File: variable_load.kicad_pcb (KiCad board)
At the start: 2 copper layers, 76.2 x 51 mm, 63 parts, among them J1 Conn_01x04, J2 LEMO, J3 Conn_01x02, J4 GS3, J5 Conn_01x04, J6 Conn_01x04, J7 Conn_01x04, Q1 NTD4858N, U1 DAC5578, U2 LM324, U3 TLV1117-33, U4 PCA9306, U5 adafruit_ft232h, U6 APD123

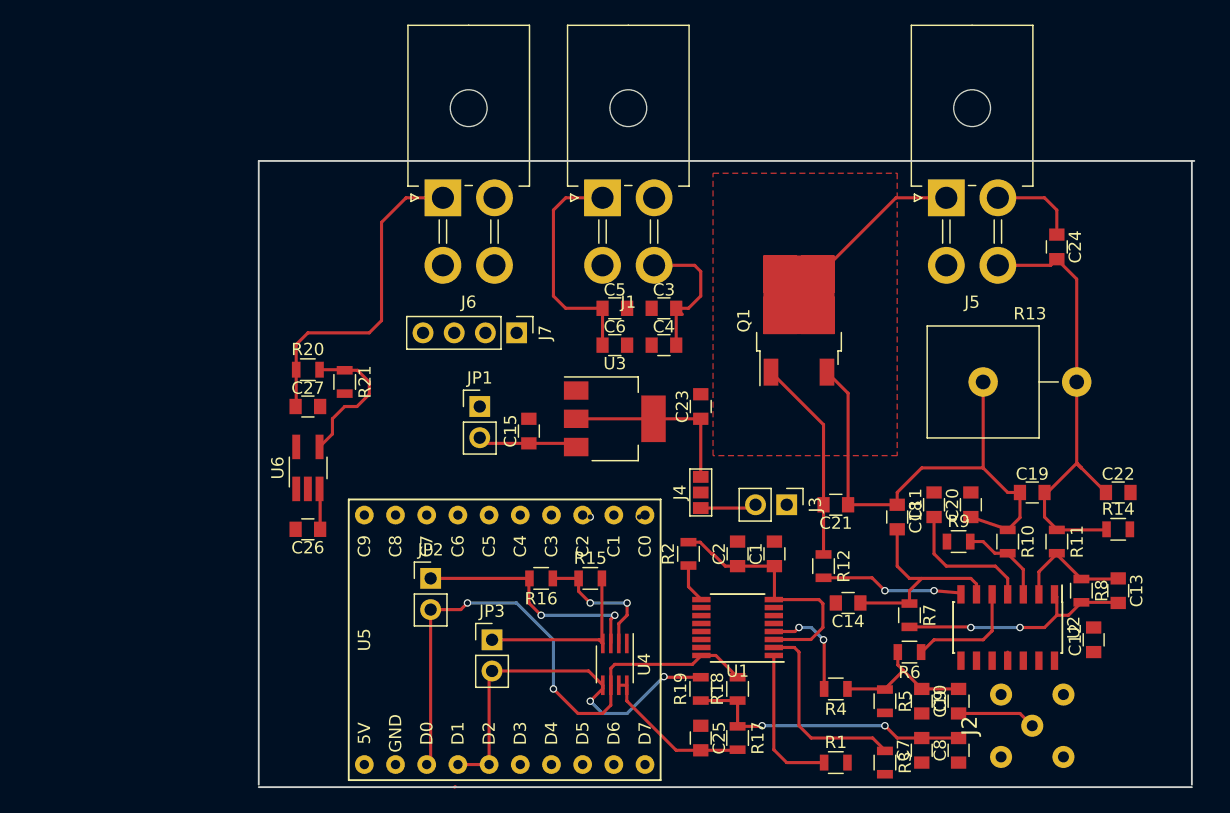
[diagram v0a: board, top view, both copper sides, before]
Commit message: pcb v3
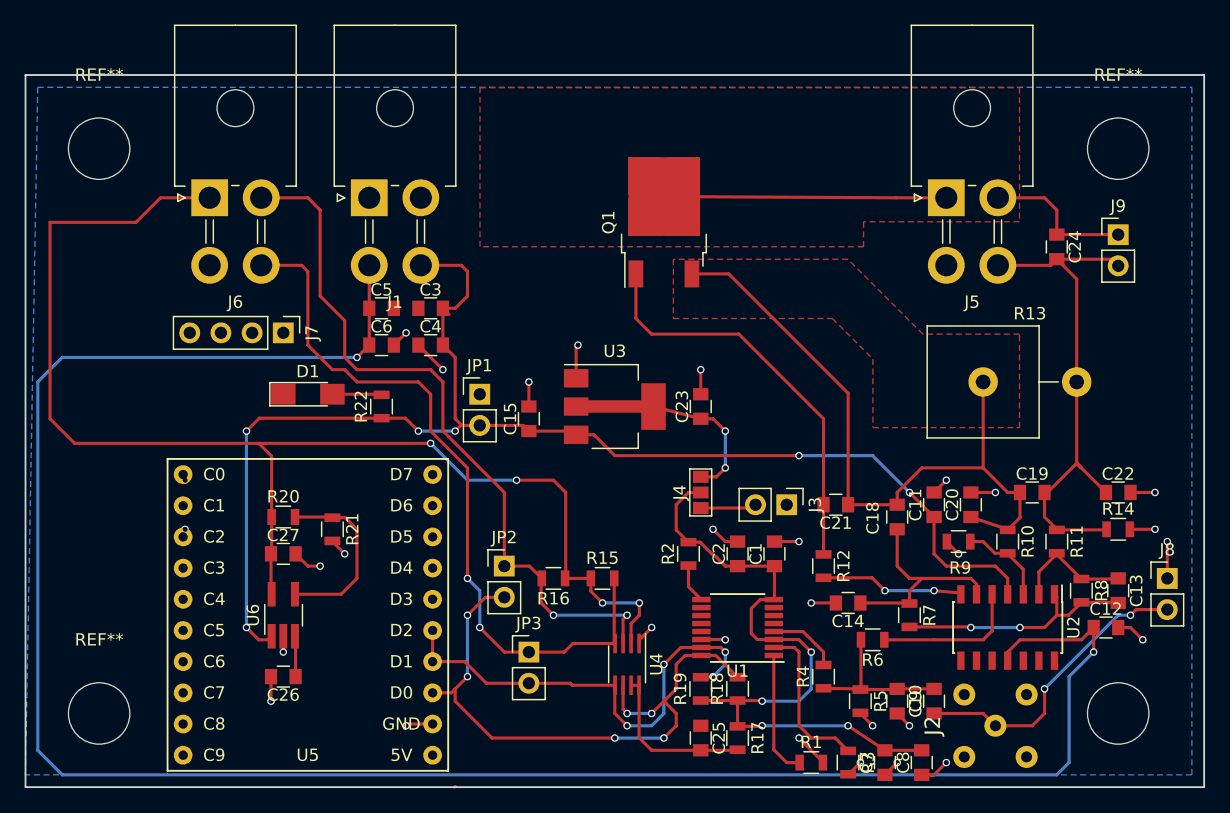
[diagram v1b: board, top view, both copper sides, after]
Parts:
- added D1: LED, LEDs:LED_1206_HandSoldering, F.Cu at (130.0, 43.0)
- added J8: Conn_01x02, Pin_Headers:Pin_Header_Straight_1x02_Pitch2.54mm, F.Cu at (200.0, 58.0)
- added J9: Conn_01x02, Pin_Headers:Pin_Header_Straight_1x02_Pitch2.54mm, F.Cu at (196.0, 30.0)
- added R22: R, Resistors_SMD:R_0805, F.Cu at (136.0, 44.0)
- added REF**: MountingHole_5mm, Mounting_Holes:MountingHole_5mm, F.Cu at (113.0, 69.0)
- added REF**: MountingHole_5mm, Mounting_Holes:MountingHole_5mm, F.Cu at (113.0, 23.0)
- added REF**: MountingHole_5mm, Mounting_Holes:MountingHole_5mm, F.Cu at (196.0, 69.0)
- added REF**: MountingHole_5mm, Mounting_Holes:MountingHole_5mm, F.Cu at (196.0, 23.0)
- moved U5 34.0 mm to (130.0, 47.0), turned to 180 degrees
- moved C3 19.0 mm to (140.0, 36.0)
- moved C4 19.0 mm to (140.0, 39.0)
- moved C5 19.0 mm to (136.0, 36.0)
- moved C6 19.0 mm to (136.0, 39.0)
- moved J1 19.0 mm to (135.0, 27.0)
- moved J6 19.0 mm to (122.0, 27.0)
- moved J7 19.0 mm to (128.0, 38.0)
- moved Q1 13.6 mm to (159.0, 29.0)
- moved C26 12.2 mm to (128.0, 66.0)
- moved C27 12.2 mm to (128.0, 56.0)
- moved R20 12.2 mm to (128.0, 53.0)
- moved U6 12.2 mm to (128.0, 61.0)
- moved R21 12.0 mm to (132.0, 54.0)
- moved JP2 6.08 mm to (146.0, 57.0)
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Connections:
- C3 pad 1: GND -> Net-(C3-Pad1)
- C5 pad 2: GND -> Net-(C5-Pad2)
- J1 pad 1: /-Vcc -> GND
- J1 pad 3: GND -> /-Vcc
- U1 pad 10: (no net) -> Net-(U1-Pad10)
- U1 pad 11: (no net) -> Net-(U1-Pad11)
- U1 pad 12: (no net) -> Net-(U1-Pad12)
- U1 pad 13: (no net) -> Net-(U1-Pad13)
- U1 pad 5: (no net) -> Net-(U1-Pad5)
- U1 pad 6: (no net) -> Net-(U1-Pad6)
- U1 pad 7: (no net) -> Net-(U1-Pad7)
- U2 pad 10: (no net) -> Net-(U2-Pad10)
- U2 pad 12: (no net) -> Net-(U2-Pad12)
- U2 pad 13: (no net) -> Net-(U2-Pad13)
- U2 pad 14: (no net) -> Net-(U2-Pad14)
- U2 pad 8: (no net) -> Net-(U2-Pad8)
- U2 pad 9: (no net) -> Net-(U2-Pad9)
- U5 pad 1: (no net) -> Net-(U5-Pad1)
- U5 pad 10: (no net) -> Net-(U5-Pad10)
- U5 pad 11: (no net) -> Net-(U5-Pad11)
- U5 pad 12: (no net) -> Net-(U5-Pad12)
- U5 pad 13: (no net) -> Net-(U5-Pad13)
- U5 pad 14: (no net) -> Net-(U5-Pad14)
- U5 pad 15: (no net) -> Net-(U5-Pad15)
- U5 pad 16: (no net) -> Net-(U5-Pad16)
- U5 pad 17: (no net) -> Net-(U5-Pad17)
- U5 pad 18: (no net) -> Net-(U5-Pad18)
- U5 pad 19: (no net) -> Net-(U5-Pad19)
- U5 pad 20: (no net) -> Net-(U5-Pad20)
- U5 pad 6: (no net) -> Net-(U5-Pad6)
- U5 pad 7: (no net) -> Net-(U5-Pad7)
- U5 pad 8: (no net) -> Net-(U5-Pad8)
- U5 pad 9: (no net) -> Net-(U5-Pad9)
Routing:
- net /-Vcc: track 19.5 -> 170.3 mm, vias 0 -> 2
- net /+Vcc: track 33.9 -> 109.8 mm, vias 0 -> 6
- net /VREF: track 38.0 -> 105.4 mm, vias 2 -> 4
- net GND: track 0.14 -> 57.1 mm, vias 0 -> 28
- net /SDA_LO: track 14.5 -> 59.9 mm, vias 0 -> 2
- net /SCL_LO: track 20.0 -> 59.3 mm
- net Net-(C9-Pad1): track 6.41 -> 24.5 mm, vias 0 -> 2
- net Net-(C21-Pad2): track 16.6 -> 33.3 mm
- net Net-(C18-Pad1): track 41.8 -> 56.1 mm
- net Net-(C24-Pad1): track 22.6 -> 35.4 mm
- net /VCC_DAC: track 44.6 -> 56.3 mm, vias 2 -> 4
- net /SDA_HI: track 32.2 -> 39.1 mm, vias 2 -> 4
- net Net-(C19-Pad2): track 38.5 -> 43.7 mm
- net Net-(D1-Pad2): track 0.00 -> 4.05 mm
- net /SCL_HI: track 49.8 -> 53.1 mm, vias 2 -> 6
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- added copper zone on B.Cu, net GND
- added copper zone on F.Cu, net Net-(C18-Pad1)
- added copper zone on F.Cu, net Net-(C24-Pad1)
- removed copper zone on F.Cu, net (none)
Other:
- board size 76.2 x 51 mm -> 96 x 58 mm
